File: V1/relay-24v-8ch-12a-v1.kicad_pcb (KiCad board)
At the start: 2 copper layers, 98 x 67.8 mm, 47 parts, among them J1 DB141V-2.54-2P, J2 DB141V-2.54-4P, J3 DB141V-2.54-4P, J4 DB142V-5.08-4P, J5 DB142V-5.08-4P, J6 DB142V-5.08-4P, J7 DB142V-5.08-4P, K1 G5PZ-1A, K2 G5PZ-1A, K3 G5PZ-1A, K4 G5PZ-1A, K5 G5PZ-1A, K6 G5PZ-1A, K7 G5PZ-1A, K8 G5PZ-1A

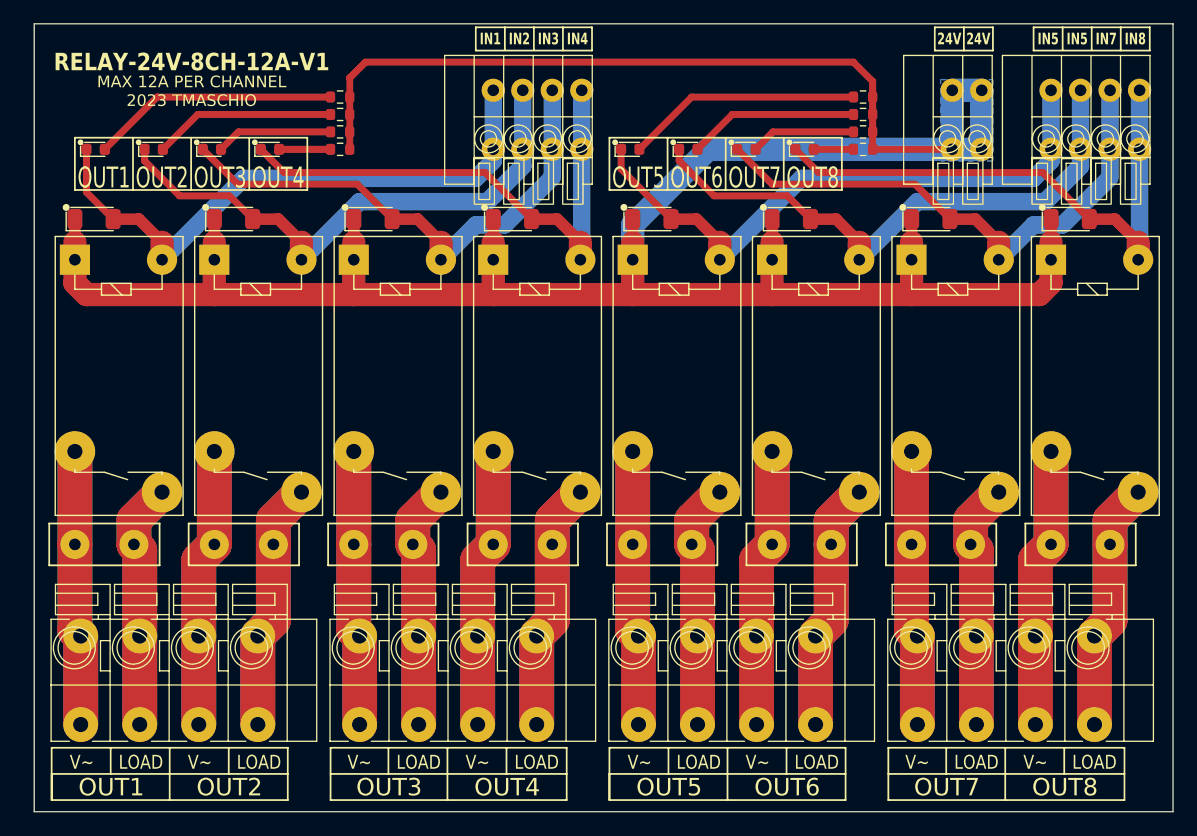
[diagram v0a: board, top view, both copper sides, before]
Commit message: Review before fabrication
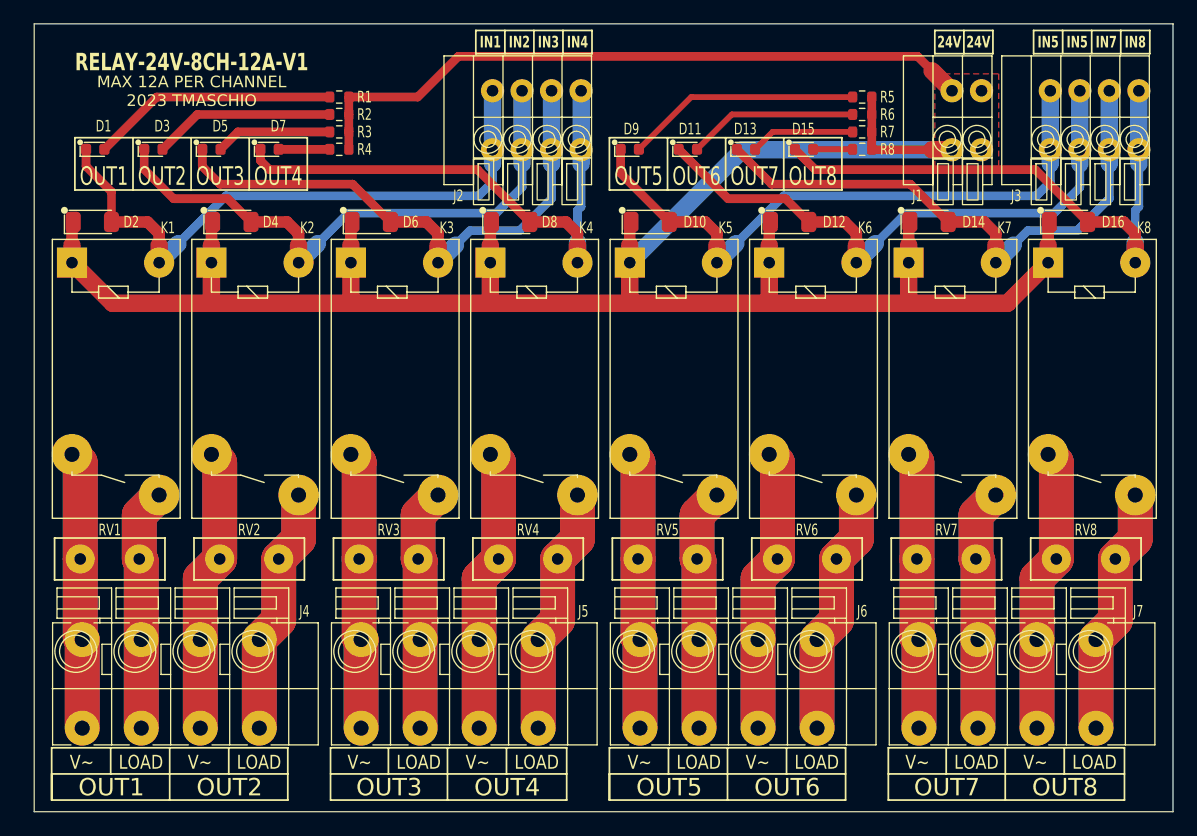
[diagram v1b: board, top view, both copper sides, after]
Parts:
- R1, R2, R3, R4, R5, R6, R7, R8: value 6k8/100mW -> 10k/100mW
- moved K1 10.8 mm to (132.0, 92.8)
- moved K2 10.8 mm to (144.0, 92.8)
- moved K3 10.8 mm to (156.0, 92.8)
- moved K4 10.8 mm to (168.0, 92.8)
- moved K5 10.8 mm to (180.0, 92.8)
- moved K6 10.8 mm to (192.0, 92.8)
- moved K7 10.8 mm to (204.0, 92.8)
- moved K8 10.8 mm to (216.0, 92.8)
- moved J4 8.50 mm to (136.8, 119.0)
- moved J5 8.50 mm to (160.8, 119.0)
- moved J6 8.50 mm to (184.8, 119.0)
- moved J7 8.50 mm to (208.8, 119.0)
- moved J2 4.65 mm to (168.2, 70.5)
- moved J3 4.65 mm to (216.2, 70.5)
- moved RV1 3.25 mm to (131.5, 108.2)
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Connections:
- net Net-(D1-A) renamed /LED1
- net Net-(D1-K) renamed /IN1
- net Net-(D10-A) renamed /IN5
- net Net-(D11-A) renamed /LED6
- net Net-(D11-K) renamed /IN6
- net Net-(D13-A) renamed /LED7
- net Net-(D13-K) renamed /IN7
- net Net-(D15-A) renamed /LED8
- net Net-(D15-K) renamed /IN8
- net Net-(D3-A) renamed /LED2
- net Net-(D3-K) renamed /IN2
- net Net-(D5-A) renamed /LED3
- net Net-(D5-K) renamed /IN3
- net Net-(D7-A) renamed /LED4
- net Net-(D7-K) renamed /IN4
- net Net-(D9-A) renamed /LED5
- net Net-(J4-Pin_1) renamed /OUT1PW
- net Net-(J4-Pin_2) renamed /OUT1LD
- net Net-(J4-Pin_3) renamed /OUT2PW
- net Net-(J4-Pin_4) renamed /OUT2LD
- net Net-(J5-Pin_1) renamed /OUT3PW
- net Net-(J5-Pin_2) renamed /OUT3LD
- net Net-(J5-Pin_3) renamed /OUT4PW
- net Net-(J5-Pin_4) renamed /OUT4LD
- net Net-(J6-Pin_1) renamed /OUT5PW
- net Net-(J6-Pin_2) renamed /OUT5LD
- net Net-(J6-Pin_3) renamed /OUT6PW
- net Net-(J6-Pin_4) renamed /OUT6LD
- net Net-(J7-Pin_1) renamed /OUT7PW
- net Net-(J7-Pin_2) renamed /OUT7LD
- net Net-(J7-Pin_3) renamed /OUT8PW
- net Net-(J7-Pin_4) renamed /OUT8LD
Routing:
- net +24V: track 248.4 -> 238.5 mm
- net /IN6: track 53.9 -> 51.0 mm
- net /IN3: track 45.2 -> 48.0 mm
- net /IN5: track 52.4 -> 54.4 mm
- net /IN1: track 51.6 -> 53.6 mm
- net /IN7: track 47.2 -> 49.1 mm
- net /IN2: track 51.9 -> 50.0 mm
- net /IN4: track 46.9 -> 48.3 mm
- net /OUT4PW: track 48.1 -> 49.1 mm
- net /OUT8PW: track 48.1 -> 49.1 mm
- net /OUT6PW: track 48.1 -> 49.1 mm
- net /OUT2PW: track 48.1 -> 49.1 mm
- net /IN8: track 48.9 -> 49.7 mm
- net /OUT7LD: track 42.4 -> 41.7 mm
- net /OUT3LD: track 42.4 -> 41.7 mm
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- added copper zone on F.Cu, net +24V
- removed copper zone on B.Cu, net +24V
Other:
- rule pad_to_mask_clearance: 0 -> 0.1
